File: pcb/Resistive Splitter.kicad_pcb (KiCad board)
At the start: 2 copper layers, 75 x 40 mm, 6 parts, among them J1 SMA 50, J2 SMA 50, J3 SMA 50

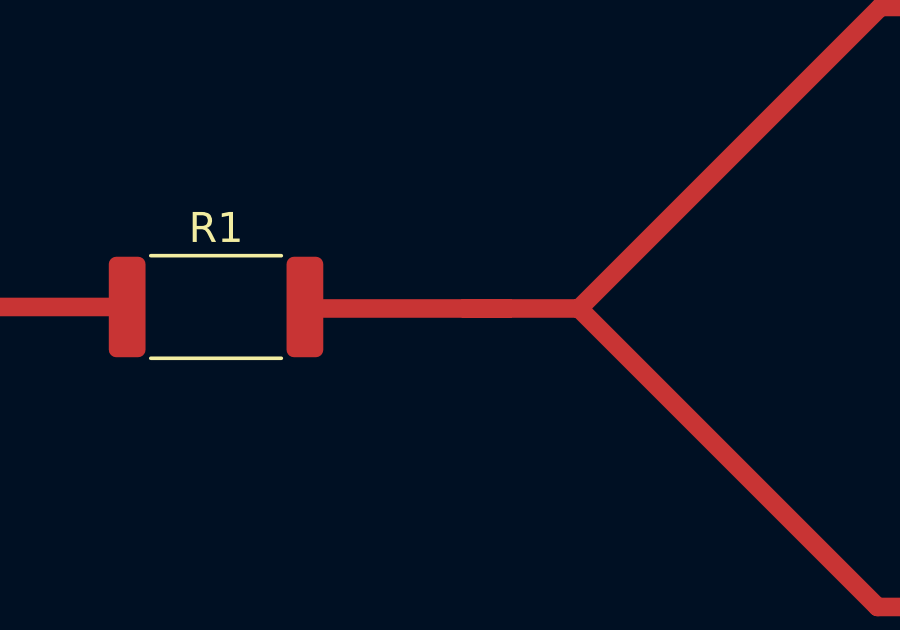
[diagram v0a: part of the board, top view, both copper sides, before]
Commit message: semmantic error
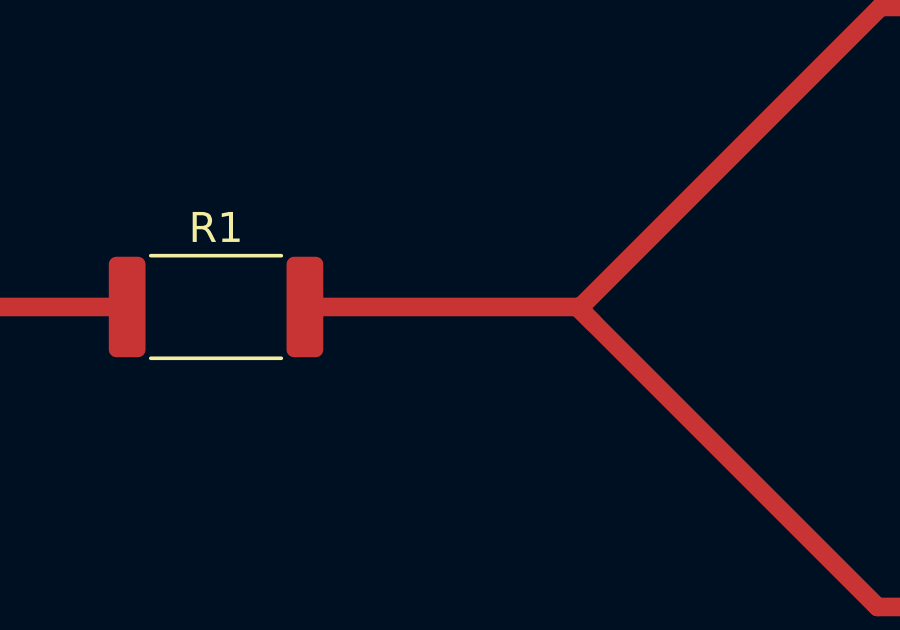
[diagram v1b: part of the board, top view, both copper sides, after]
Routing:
- net Net-(R1-Pad2): track 42.6 -> 41.8 mm
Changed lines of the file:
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@@
 		)
+	)
+	(segment
+		(start 69.905 10)
+		(end 52.9625 10)
+		(width 0.62)
+		(layer "F.Cu")
+		(net "Net-(J2-In)")
 	)
 	(via
@@
 		(filling no)
 		(net "GND")
+	)
+	(segment
+		(start 35.15 20.05)
+		(end 45.1 30)
+		(width 0.62)
+		(layer "F.Cu")
+		(net "Net-(R1-Pad2)")
+	)
+	(segment
+		(start 47 30)
+		(end 45.9 30)
+		(width 0.62)
+		(layer "F.Cu")
+		(net "Net-(R1-Pad2)")
+	)
+	(segment
+		(start 47 10)
+		(end 45.2 10)
+		(width 0.62)
+		(layer "F.Cu")
+		(net "Net-(R1-Pad2)")
+	)
+	(segment
+		(start 45.1 30)
+		(end 45.9 30)
+		(width 0.62)
+		(layer "F.Cu")
+		(net "Net-(R1-Pad2)")
+	)
+	(segment
+		(start 26.0625 20.05)
+		(end 26.0125 20)
+		(width 0.62)
+		(layer "F.Cu")
+		(net "Net-(R1-Pad2)")
+	)
+	(segment
+		(start 45.2 10)
+		(end 35.15 20.05)
+		(width 0.62)
+		(layer "F.Cu")
+		(net "Net-(R1-Pad2)")
+	)
+	(segment
+		(start 35.1 20)
+		(end 26.0625 20)
+		(width 0.62)
+		(layer "F.Cu")
+		(net "Net-(R1-Pad2)")
+	)
+	(segment
+		(start 35.635 20.535)
+		(end 35.1 20)
+		(width 0.62)
+		(layer "F.Cu")
+		(net "Net-(R1-Pad2)")
+	)
+	(segment
+		(start 70.905 30)
+		(end 52.9625 30)
+		(width 0.62)
+		(layer "F.Cu")
+		(net "Net-(J3-In)")
 	)
 	(segment
@@
 		(net "Net-(J1-In)")
 	)
-	(segment
-		(start 69.905 10)
-		(end 52.9625 10)
-		(width 0.62)
-		(layer "F.Cu")
-		(net "Net-(J2-In)")
-	)
-	(segment
-		(start 70.905 30)
-		(end 52.9625 30)
-		(width 0.62)
-		(layer "F.Cu")
-		(net "Net-(J3-In)")
-	)
-	(segment
-		(start 35.15 20.05)
-		(end 45.1 30)
-		(width 0.62)
-		(layer "F.Cu")
-		(net "Net-(R1-Pad2)")
-	)
-	(segment
-		(start 47 30)
-		(end 45.9 30)
-		(width 0.62)
-		(layer "F.Cu")
-		(net "Net-(R1-Pad2)")
-	)
-	(segment
-		(start 47 10)
-		(end 45.2 10)
-		(width 0.62)
-		(layer "F.Cu")
-		(net "Net-(R1-Pad2)")
-	)
-	(segment
-		(start 45.1 30)
-		(end 45.9 30)
-		(width 0.62)
-		(layer "F.Cu")
-		(net "Net-(R1-Pad2)")
-	)
-	(segment
-		(start 26.0625 20.05)
-		(end 26.0125 20)
-		(width 0.62)
-		(layer "F.Cu")
-		(net "Net-(R1-Pad2)")
-	)
-	(segment
-		(start 31.35 20.05)
-		(end 26.0625 20.05)
-		(width 0.62)
-		(layer "F.Cu")
-		(net "Net-(R1-Pad2)")
-	)
-	(segment
-		(start 45.2 10)
-		(end 35.15 20.05)
-		(width 0.62)
-		(layer "F.Cu")
-		(net "Net-(R1-Pad2)")
-	)
-	(segment
-		(start 31.35 20.05)
-		(end 32.8 20.05)
-		(width 0.62)
-		(layer "F.Cu")
-		(net "Net-(R1-Pad2)")
-	)
-	(segment
-		(start 35.15 20.05)
-		(end 31.35 20.05)
-		(width 0.62)
-		(layer "F.Cu")
-		(net "Net-(R1-Pad2)")
-	)
 	(zone

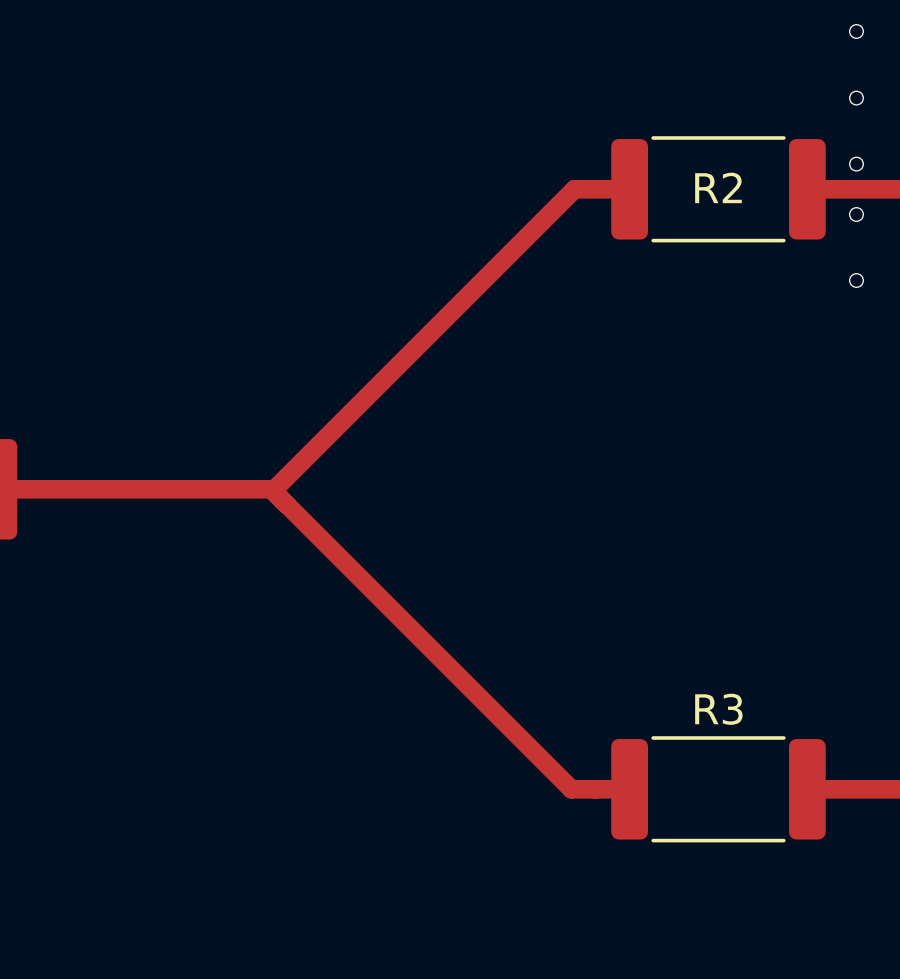
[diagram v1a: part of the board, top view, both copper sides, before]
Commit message: pcb update
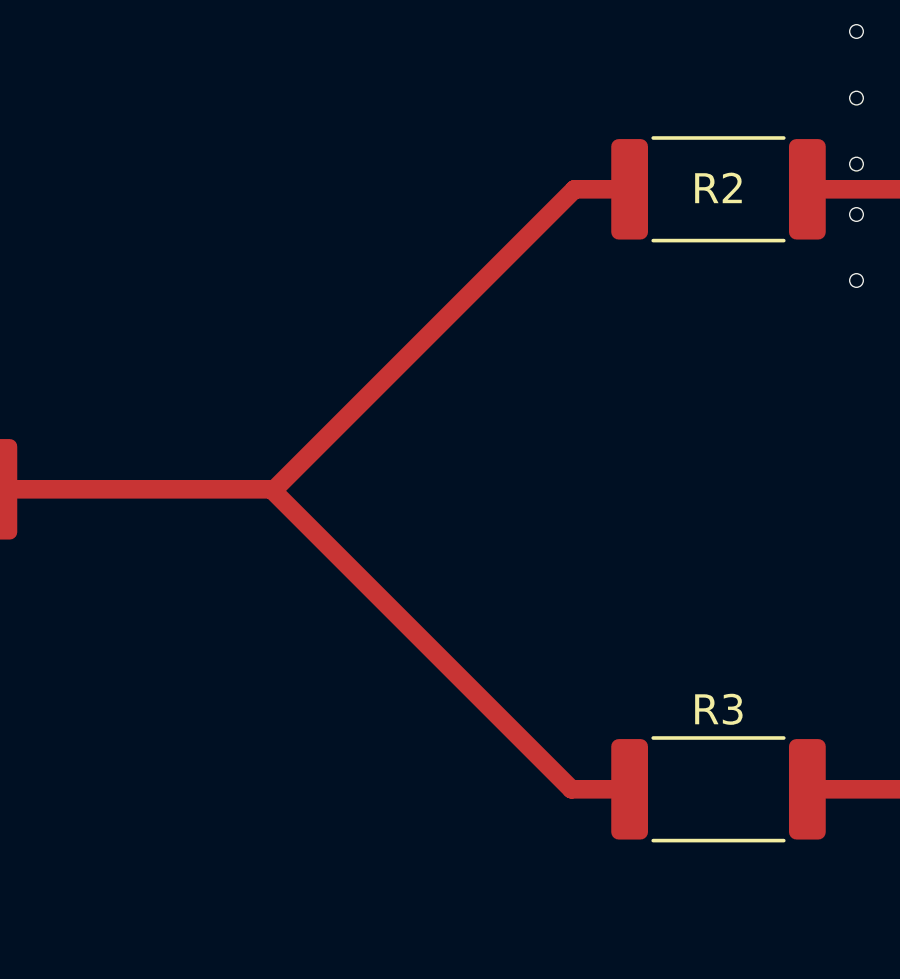
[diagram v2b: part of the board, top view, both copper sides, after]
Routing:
- net Net-(R1-Pad2): track 41.8 -> 41.2 mm
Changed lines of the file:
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@@
 	)
 	(segment
-		(start 35.15 20.05)
-		(end 45.1 30)
+		(start 35.2 20)
+		(end 35.1 20)
 		(width 0.62)
 		(layer "F.Cu")
@@
 	)
 	(segment
-		(start 47 30)
-		(end 45.9 30)
-		(width 0.62)
-		(layer "F.Cu")
-		(net "Net-(R1-Pad2)")
-	)
-	(segment
-		(start 47 10)
-		(end 45.2 10)
-		(width 0.62)
-		(layer "F.Cu")
-		(net "Net-(R1-Pad2)")
-	)
-	(segment
-		(start 45.1 30)
-		(end 45.9 30)
+		(start 35.1 20)
+		(end 45.1 30)
 		(width 0.62)
 		(layer "F.Cu")
@@
 	)
 	(segment
-		(start 45.2 10)
-		(end 35.15 20.05)
-		(width 0.62)
-		(layer "F.Cu")
-		(net "Net-(R1-Pad2)")
-	)
-	(segment
 		(start 35.1 20)
 		(end 26.0625 20)
@@
 	)
 	(segment
-		(start 35.635 20.535)
-		(end 35.1 20)
+		(start 45.2 10)
+		(end 35.2 20)
 		(width 0.62)
 		(layer "F.Cu")
+		(net "Net-(R1-Pad2)")
+	)
+	(segment
+		(start 45.1 30)
+		(end 47 30)
+		(width 0.62)
+		(layer "F.Cu")
+		(net "Net-(R1-Pad2)")
+	)
+	(segment
+		(start 47 10)
+		(end 45.2 10)
+		(width 0.62)
+		(layer "F.Cu")
